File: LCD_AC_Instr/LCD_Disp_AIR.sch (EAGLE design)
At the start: 30 parts, among them J1 12V input, Q1 16MHz, SW1 ENCODER_SW1-PEC12, U1 ATMEGA328P, U2 5V, U3 +5V

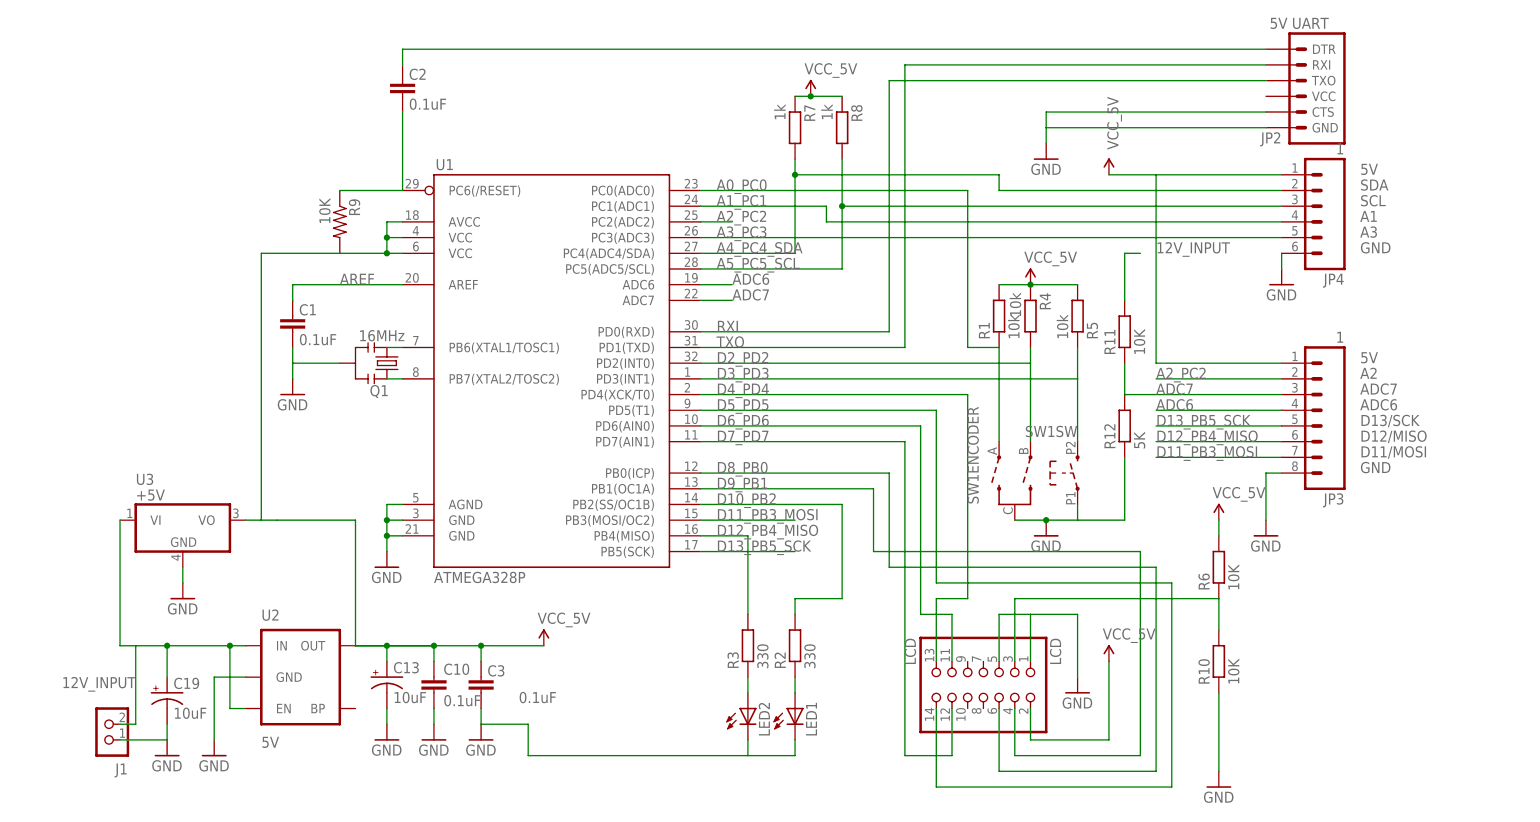
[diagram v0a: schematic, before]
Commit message: Revised to rev 0.1
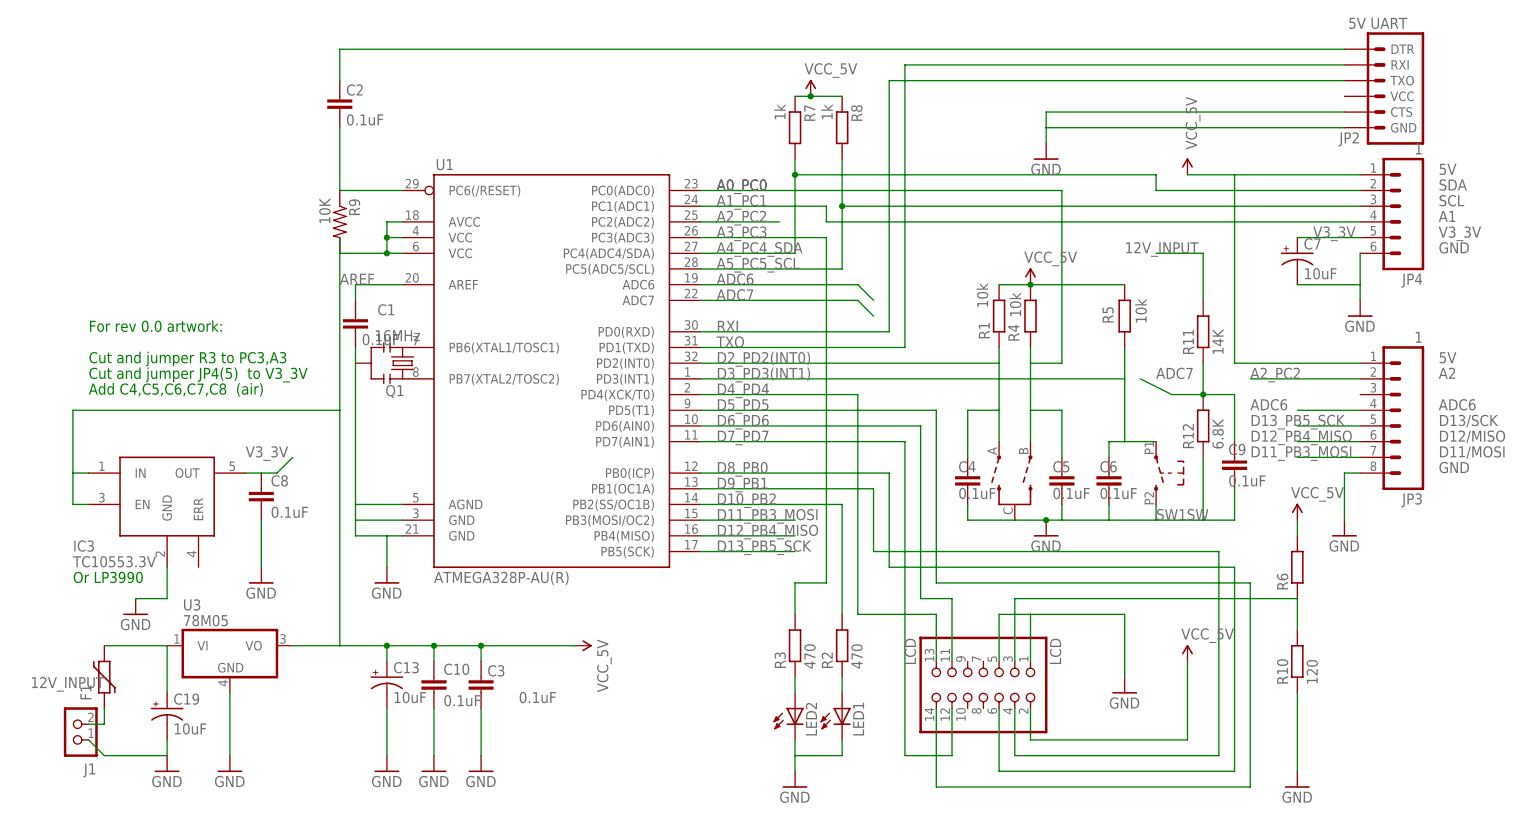
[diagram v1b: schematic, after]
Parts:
- removed U2: 5V, SparkFun:V_REG_LDOSMD
- added C4, C5, C6, C8, C9: 0.1uF, SparkFun:CAP0805
- added C7: 10uF, SparkFun:CAP_POL1206
- added F1: (no value), dp_devices:FUSE_PTC-0805
- added IC3: TC10553.3V, 1AA_Stofer:TC10553.3V
- C1, C10, C2, C3: device SparkFun:CAP0402 -> SparkFun:CAP0805
- C19: device SparkFun:CAP_POL1206 -> SparkFun:CAP_POL7343
- R10: value 10K -> 120
- R11: value 10K -> 14K
- R12: value 5K -> 6.8K
- R2, R3: value 330 -> 470
- R6: value 10K -> (none)
- R9: device SparkFun:RESISTOR0402 -> SparkFun:RESISTOR0603
- U1: value ATMEGA328P -> ATMEGA328P-AU(R)
- U3: value +5V -> 78M05
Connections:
- removed net D2_PD2: R4.2, SW1ENCODER.B, U1.PD2(INT0)
- removed net D3_PD3: R5.1, SW1SW.2, U1.PD3(INT1)
- new net D2_PD2(INT0): C4.2, R1.1, SW1ENCODER.A, U1.PD2(INT0)
- new net D3_PD3(INT1): C6.2, R5.1, SW1SW.1, U1.PD3(INT1)
- new net N$11: F1.1, J1.2
- new net V3_3V: C7.+, C8.1, IC3.OUT, JP4.5
- net 12V_INPUT: now also F1.2; no longer J1.2, U2.EN, U2.IN
- net 5V: now also IC3.EN, IC3.IN; no longer U2.OUT
- net A0_PC0: now also C5.2, R4.2, SW1ENCODER.B; no longer R1.1, SW1ENCODER.A
- net A3_PC3: now also R3.2; no longer JP4.5
- net ADC7: now also C9.1; no longer JP3.3
- net D12_PB4_MISO: no longer R3.2
- net GND: now also C4.1, C5.1, C6.1, C7.-, C8.2, C9.2, IC3.GND, SW1SW.2; no longer SW1SW.1, U2.GND
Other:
- note added: "Add C4,C5,C6,C7,C8 (air)"
- note added: "Cut and jumper JP4(5) to V3_3V"
- note added: "Cut and jumper R3 to PC3,A3"
- note added: "For rev 0.0 artwork:"
- note added: "Or LP3990"
- note removed: "A3"
- note removed: "ADC7"
- moved on the sheet: C1, C19, C2, J1, JP2, JP3, JP4, LED1, LED2, Q1, R10, R11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
